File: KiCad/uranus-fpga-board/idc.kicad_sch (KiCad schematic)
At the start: 1 part, among them J2 1040100018

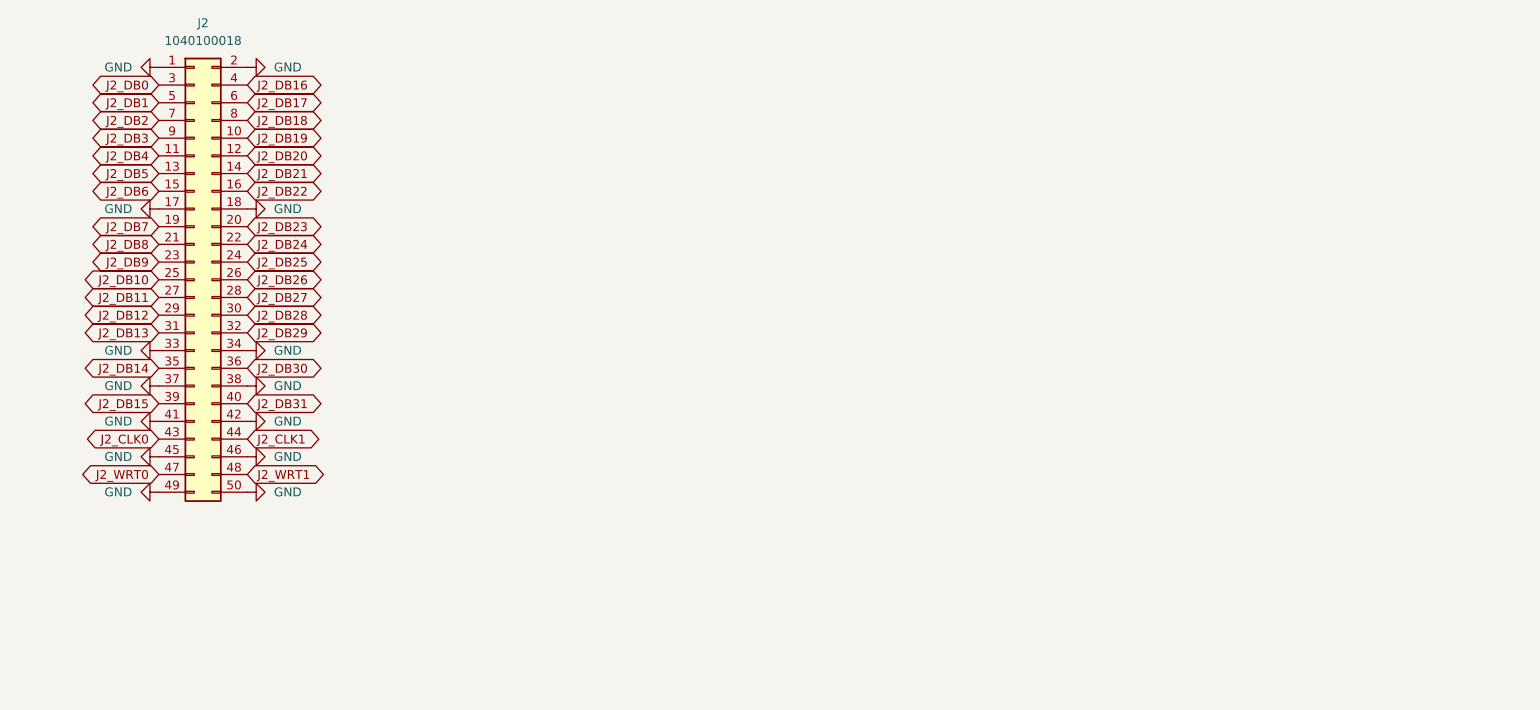
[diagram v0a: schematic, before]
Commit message: big things happening in schematic quality
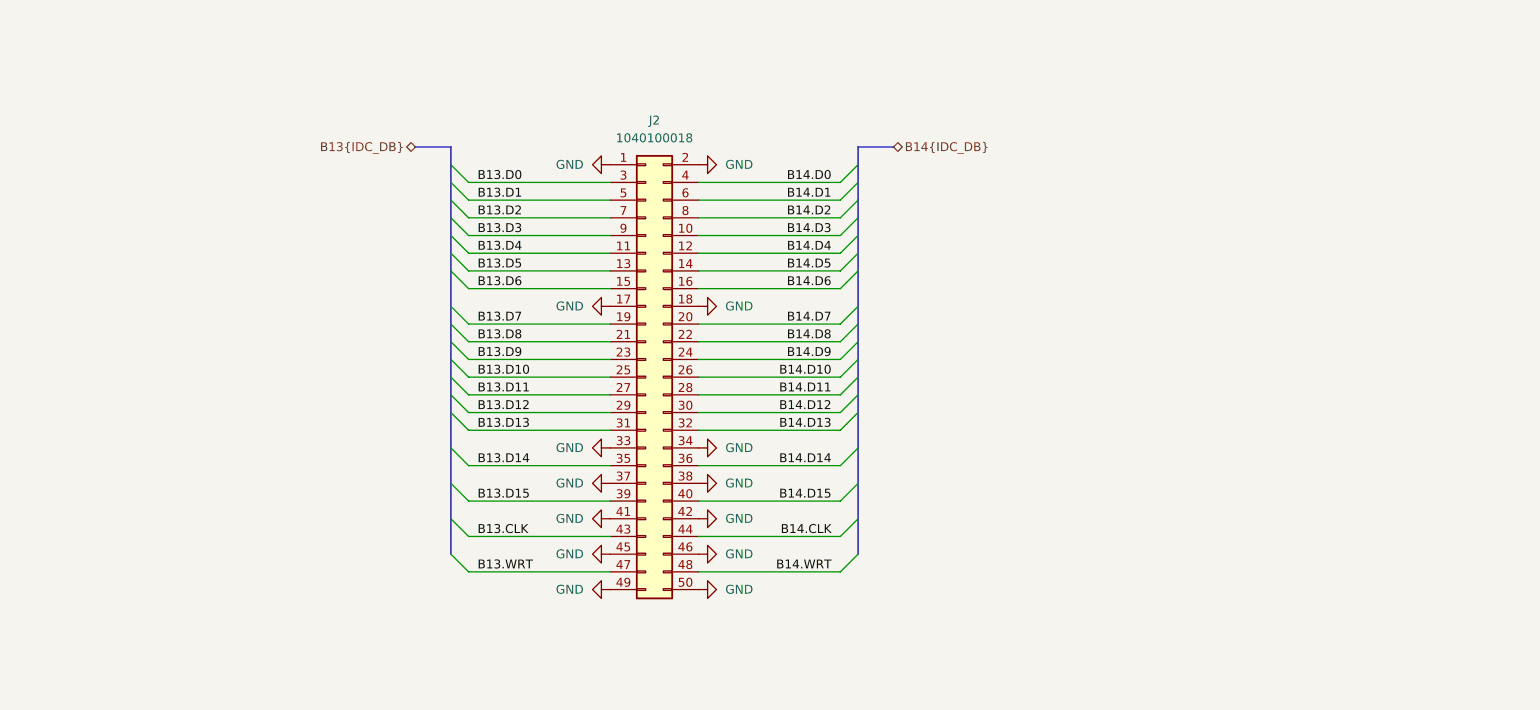
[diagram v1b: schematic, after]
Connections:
- net J2_CLK0 renamed B13.CLK
- net J2_CLK1 renamed B14.CLK
- net J2_DB0 renamed B13.D0
- net J2_DB1 renamed B13.D1
- net J2_DB10 renamed B13.D10
- net J2_DB11 renamed B13.D11
- net J2_DB12 renamed B13.D12
- net J2_DB13 renamed B13.D13
- net J2_DB14 renamed B13.D14
- net J2_DB15 renamed B13.D15
- net J2_DB16 renamed B14.D0
- net J2_DB17 renamed B14.D1
- net J2_DB18 renamed B14.D2
- net J2_DB19 renamed B14.D3
- net J2_DB2 renamed B13.D2
- net J2_DB20 renamed B14.D4
- net J2_DB21 renamed B14.D5
- net J2_DB22 renamed B14.D6
- net J2_DB23 renamed B14.D7
- net J2_DB24 renamed B14.D8
- net J2_DB25 renamed B14.D9
- net J2_DB26 renamed B14.D10
- net J2_DB27 renamed B14.D11
- net J2_DB28 renamed B14.D12
- net J2_DB29 renamed B14.D13
- net J2_DB3 renamed B13.D3
- net J2_DB30 renamed B14.D14
- net J2_DB31 renamed B14.D15
- net J2_DB4 renamed B13.D4
- net J2_DB5 renamed B13.D5
- net J2_DB6 renamed B13.D6
- net J2_DB7 renamed B13.D7
- net J2_DB8 renamed B13.D8
- net J2_DB9 renamed B13.D9
- net J2_WRT0 renamed B13.WRT
- net J2_WRT1 renamed B14.WRT
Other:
- moved on the sheet: J2

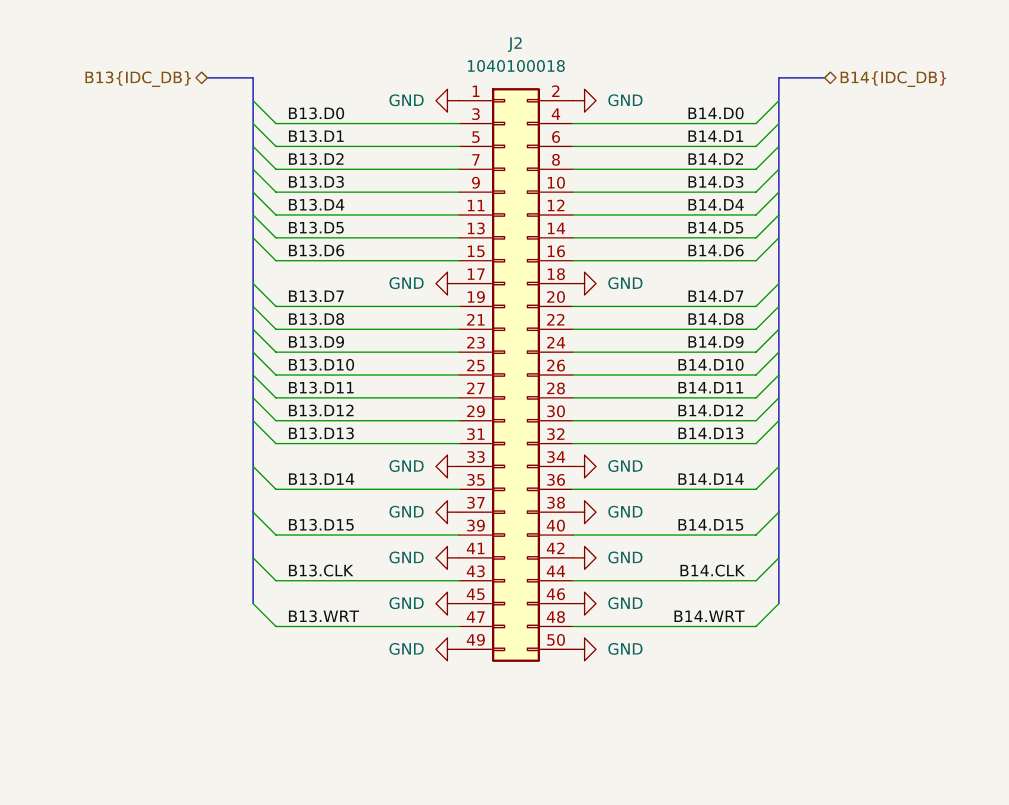
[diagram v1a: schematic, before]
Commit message: Big things have mostly happened in schematic quality
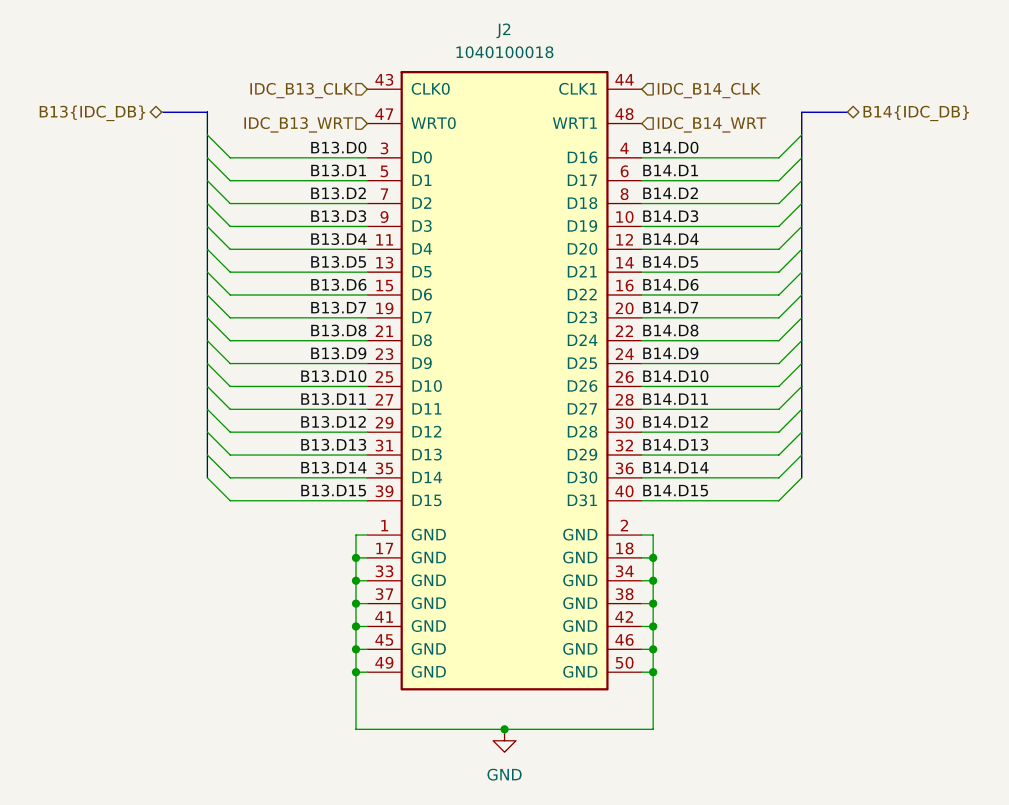
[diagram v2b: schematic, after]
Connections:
- net B13.CLK renamed IDC_B13_CLK
- net B13.WRT renamed IDC_B13_WRT
- net B14.CLK renamed IDC_B14_CLK
- net B14.WRT renamed IDC_B14_WRT
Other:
- moved on the sheet: J2

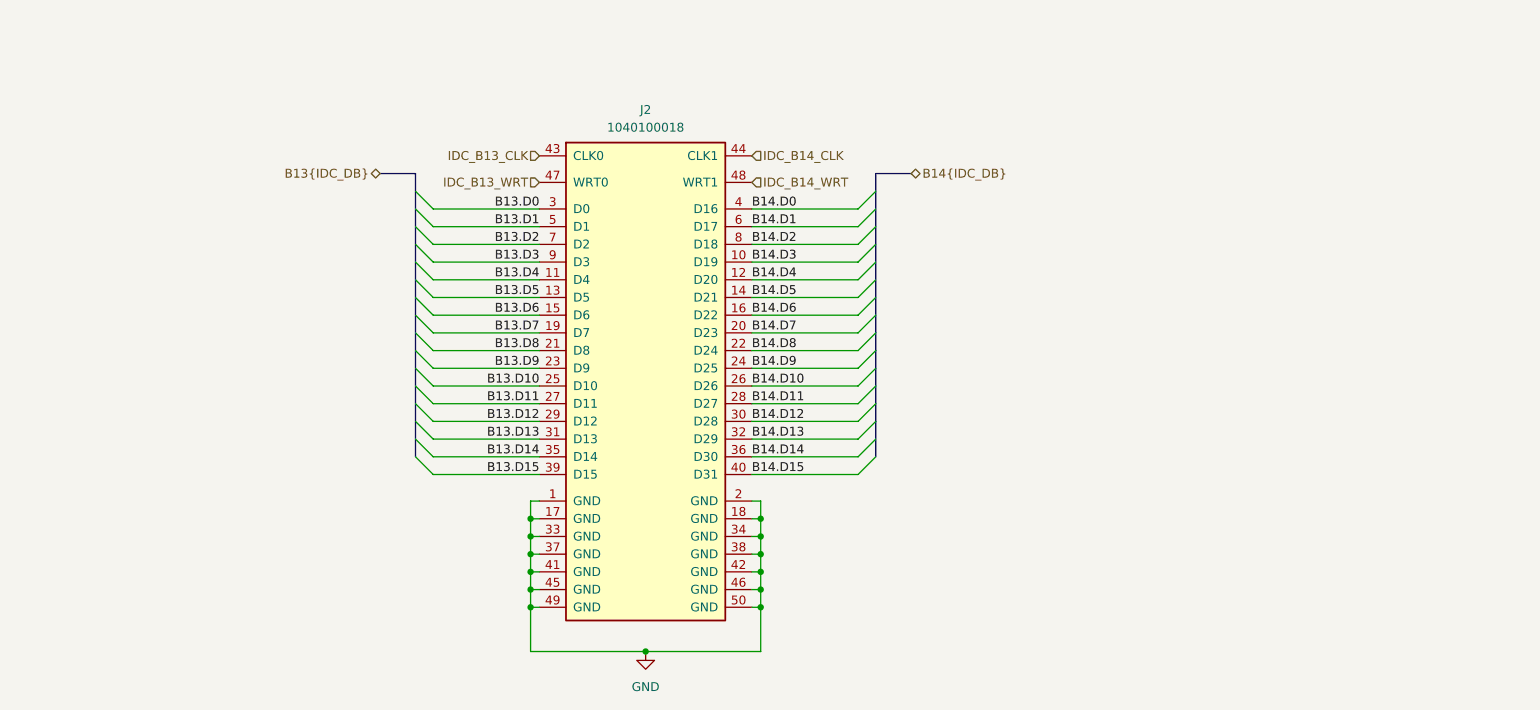
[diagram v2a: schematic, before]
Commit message: I finally did it
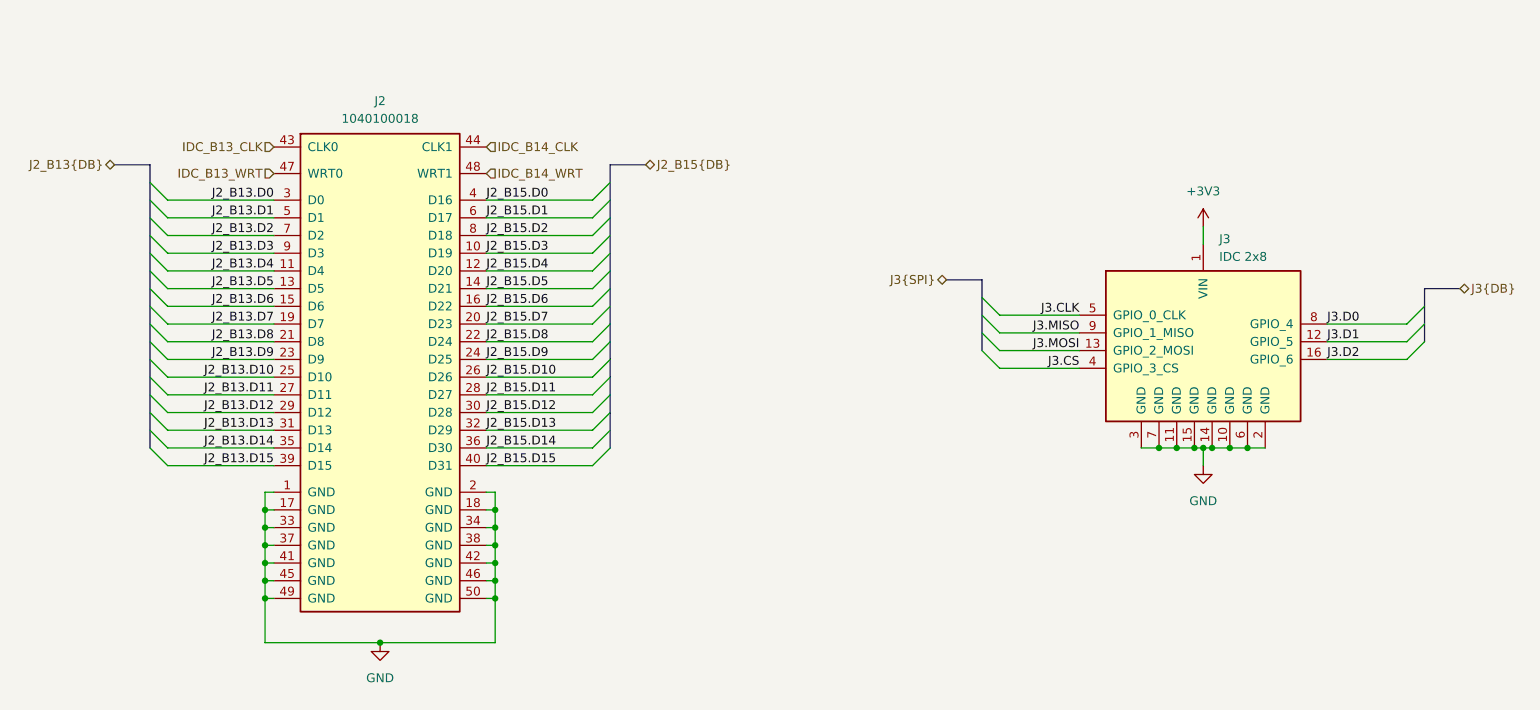
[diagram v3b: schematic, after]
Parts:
- added J3: IDC 2x8, Connector_IDC:IDC-Header_2x08_P2.54mm_Vertical_SMD, symbol Connector_Generic:Conn_02x08_Odd_Even
- J2: footprint Connector_PinHeader_1.27mm:PinHeader_2x25_P1.27mm_Vertical_SMD -> Connector_IDC:IDC-Header_2x25_P2.54mm_Vertical_SMD
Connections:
- net GND: now also J3.10 (GND), J3.11 (GND), J3.14 (GND), J3.15 (GND), J3.2 (GND), J3.3 (GND), J3.6 (GND), J3.7 (GND)
- net B13.D0 renamed J2_B13.D0
- net B13.D1 renamed J2_B13.D1
- net B13.D10 renamed J2_B13.D10
- net B13.D11 renamed J2_B13.D11
- net B13.D12 renamed J2_B13.D12
- net B13.D13 renamed J2_B13.D13
- net B13.D14 renamed J2_B13.D14
- net B13.D15 renamed J2_B13.D15
- net B13.D2 renamed J2_B13.D2
- net B13.D3 renamed J2_B13.D3
- net B13.D4 renamed J2_B13.D4
- net B13.D5 renamed J2_B13.D5
- net B13.D6 renamed J2_B13.D6
- net B13.D7 renamed J2_B13.D7
- net B13.D8 renamed J2_B13.D8
- net B13.D9 renamed J2_B13.D9
- net B14.D0 renamed J2_B15.D0
- net B14.D1 renamed J2_B15.D1
- net B14.D10 renamed J2_B15.D10
- net B14.D11 renamed J2_B15.D11
- net B14.D12 renamed J2_B15.D12
- net B14.D13 renamed J2_B15.D13
- net B14.D14 renamed J2_B15.D14
- net B14.D15 renamed J2_B15.D15
- net B14.D2 renamed J2_B15.D2
- net B14.D3 renamed J2_B15.D3
- net B14.D4 renamed J2_B15.D4
- net B14.D5 renamed J2_B15.D5
- net B14.D6 renamed J2_B15.D6
- net B14.D7 renamed J2_B15.D7
- net B14.D8 renamed J2_B15.D8
- net B14.D9 renamed J2_B15.D9
- new net +3V3: J3.1 (VIN)
- new net J3.CLK: J3.5 (GPIO_0_CLK)
- new net J3.CS: J3.4 (GPIO_3_CS)
- new net J3.D0: J3.8 (GPIO_4)
- new net J3.D1: J3.12 (GPIO_5)
- new net J3.D2: J3.16 (GPIO_6)
- new net J3.MISO: J3.9 (GPIO_1_MISO)
- new net J3.MOSI: J3.13 (GPIO_2_MOSI)
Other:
- moved on the sheet: J2
